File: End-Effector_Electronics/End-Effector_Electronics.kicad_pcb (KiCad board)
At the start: 2 copper layers, 65 x 57 mm, 48 parts, among them J1 Raspberry_Pi_2_3, J10 SW_Push_Open, J11 SW_Push_Open, J2 LynxServo, J3 LynxServo, J4 QWIIC_Generic_Conn, J5 Conn_02x05_Odd_Even, J9 SW_Push_Open, Q1 Q_PMOS_GSD, Q2 DMMT3906, Q3 Q_NMOS_GSD, Q4 Q_NMOS_GSD, Q5 Q_NMOS_GSD, U1 CAT24C32, U2 TDK_I3A4W008A033V, U3 LM22676MR-5

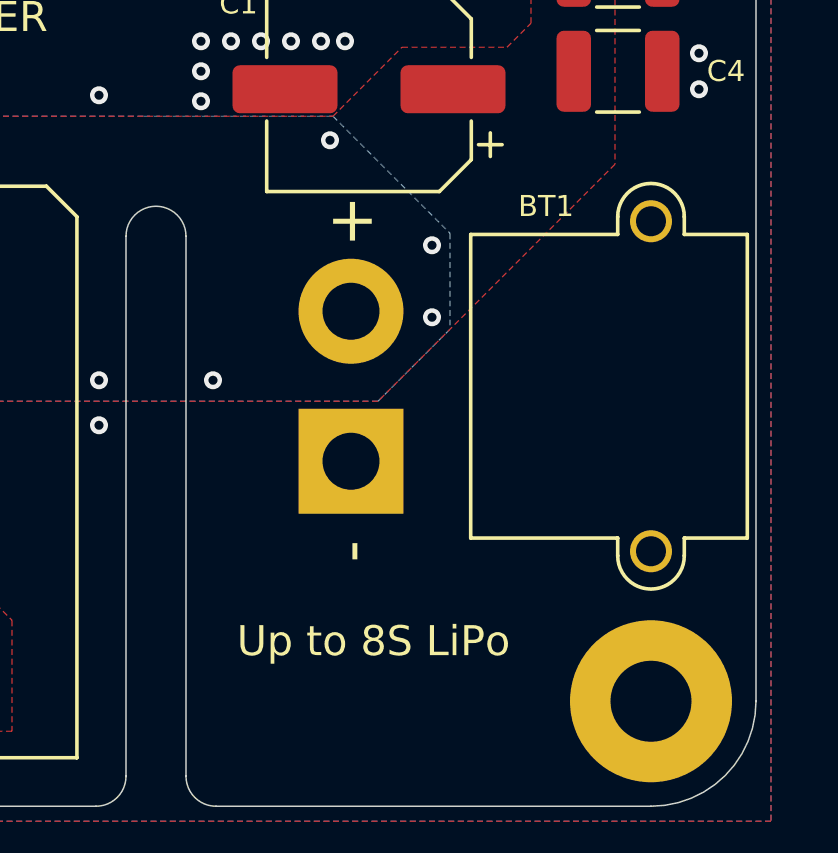
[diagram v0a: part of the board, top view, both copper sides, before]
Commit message: Fixed errors
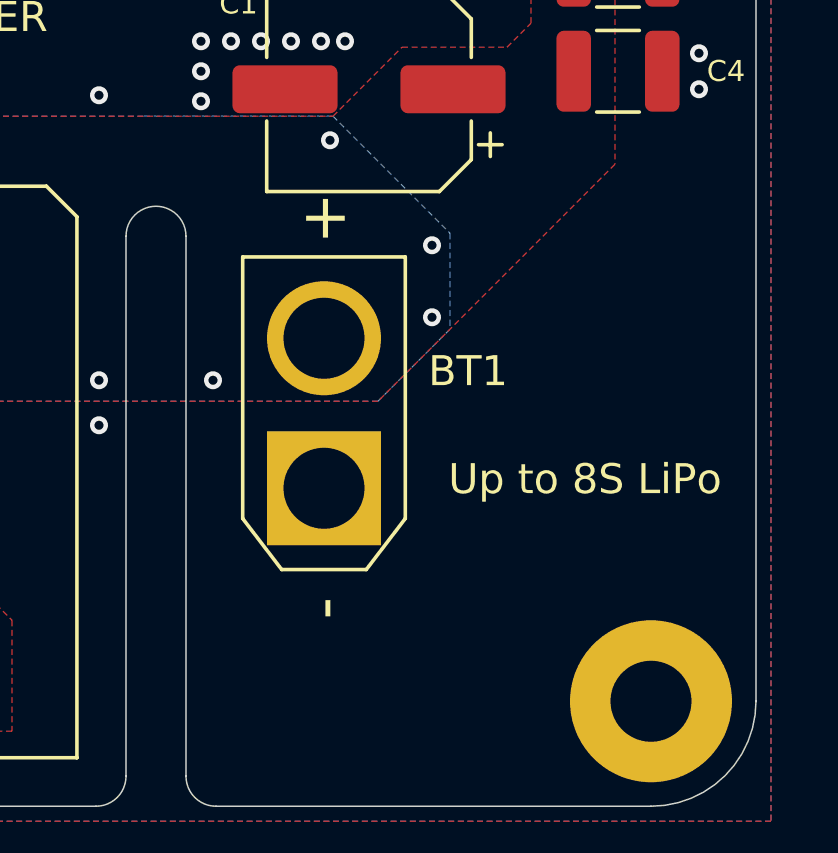
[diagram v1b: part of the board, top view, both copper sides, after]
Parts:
- BT1: footprint Connector_AMASS:AMASS_XT30PW-M_1x02_P2.50mm_Horizontal -> Connector_AMASS:AMASS_XT30U-M_1x02_P5.0mm_Vertical
- moved BT1 1.27 mm to (213.7, 124.5), turned to 90 degrees

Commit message: I changed something I guess?
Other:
- board text added: "M2.5 x4"
